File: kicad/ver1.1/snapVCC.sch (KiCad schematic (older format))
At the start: 16 parts, among them J1 Jumper Shunt, P1 CONN_01X03, P2 CONN_01X02, Q1 IRLML9301TRPbF, U1 TPS560200

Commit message: updated PCB
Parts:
- P1: footprint snapVCC_lib:3P-1.27 -> Connect:PINHEAD1-3
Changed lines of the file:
@@
 LIBS:contrib
 LIBS:valves
-LIBS:snapVCC
-LIBS:snapVCC-cache
+LIBS:bb
+LIBS:blinky-cache
 EELAYER 25 0
 EELAYER END
@@
 F 0 "P1" H 7000 4900 50  0000 C CNN
 F 1 "CONN_01X03" V 7100 4700 50  0001 C CNN
-F 2 "snapVCC_lib:3P-1.27" H 7000 4700 60  0001 C CNN
+F 2 "Connect:PINHEAD1-3" H 7000 4700 60  0001 C CNN
 F 3 "" H 7000 4700 60  0000 C CNN
 F 4 "1.27 mm pitch, male" H 7000 4700 60  0001 C CNN "Characteristics"

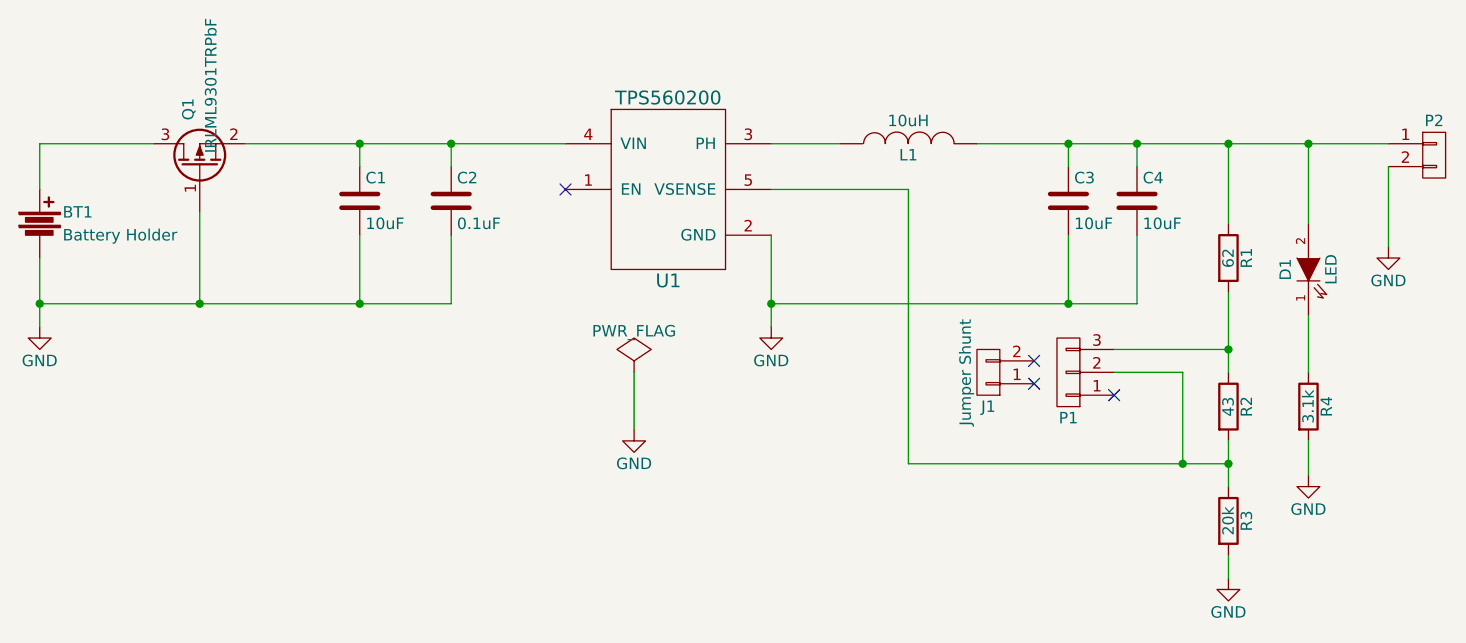
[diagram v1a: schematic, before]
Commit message: updated PCB
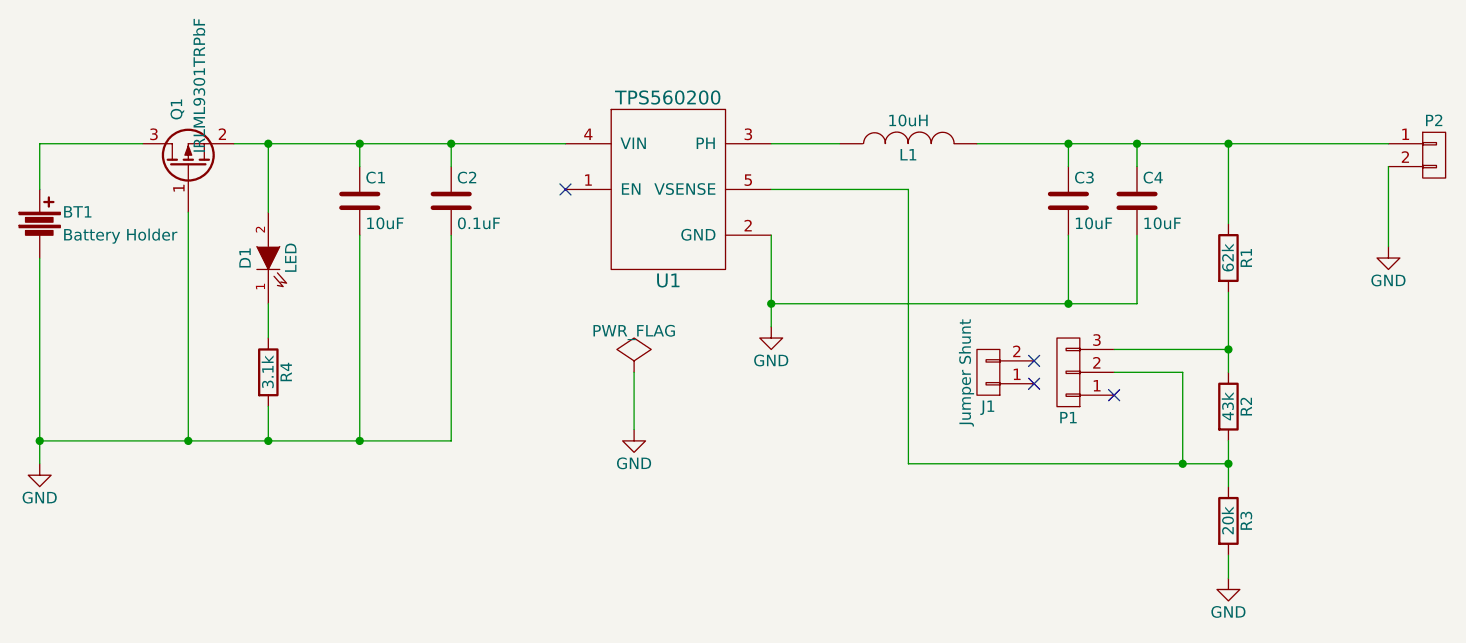
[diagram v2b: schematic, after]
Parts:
- R1: value 62 -> 62k
- R2: value 43 -> 43k
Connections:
- net at C1.1, C2.1, Q1.2 (S)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: now also D1.2 (A)
- net at C3.1, C4.1, L1.2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: no longer D1.2 (A)
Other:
- moved on the sheet: D1, Q1, R4
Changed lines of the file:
@@
 LIBS:contrib
 LIBS:valves
-LIBS:bb
-LIBS:blinky-cache
+LIBS:snapVCC
+LIBS:snapVCC-cache
 EELAYER 25 0
 EELAYER END
@@
 L Q_PMOS_GSD Q1
 U 1 1 56012F07
-P 3200 3800
-F 0 "Q1" H 3500 3850 50  0000 R CNN
-F 1 "IRLML9301TRPbF" H 3850 3750 50  0000 R CNN
-F 2 "snapVCC_lib:SOT23" H 3400 3900 29  0001 C CNN
-F 3 "" H 3200 3800 60  0000 C CNN
-F 4 "International Rectifier" H 3200 3800 60  0001 C CNN "MFN"
-F 5 "IRLML9301TRPbF" H 3200 3800 60  0001 C CNN "MFP"
-F 6 "Value" H 3200 3800 60  0001 C CNN "Link1"
-	1    3200 3800
+P 3150 3800
+F 0 "Q1" H 3450 3850 50  0000 R CNN
+F 1 "IRLML9301TRPbF" H 3800 3750 50  0000 R CNN
+F 2 "snapVCC_lib:SOT23" H 3350 3900 29  0001 C CNN
+F 3 "" H 3150 3800 60  0000 C CNN
+F 4 "International Rectifier" H 3150 3800 60  0001 C CNN "MFN"
+F 5 "IRLML9301TRPbF" H 3150 3800 60  0001 C CNN "MFP"
+F 6 "Value" H 3150 3800 60  0001 C CNN "Link1"
+	1    3150 3800
 	0    -1   -1   0
 $EndComp
@@
 P 7700 4200
 F 0 "R1" V 7780 4200 50  0000 C CNN
-F 1 "62" V 7700 4200 50  0000 C CNN
+F 1 "62k" V 7700 4200 50  0000 C CNN
 F 2 "snapVCC_lib:0603-RES" V 7630 4200 30  0001 C CNN
 F 3 "" H 7700 4200 30  0000 C CNN
@@
 P 7700 4850
 F 0 "R2" V 7780 4850 50  0000 C CNN
-F 1 "43" V 7700 4850 50  0000 C CNN
+F 1 "43k" V 7700 4850 50  0000 C CNN
 F 2 "snapVCC_lib:0603-RES" V 7630 4850 30  0001 C CNN
 F 3 "" H 7700 4850 30  0000 C CNN
@@
 L GND #PWR02
 U 1 1 56014277
-P 2500 4500
-F 0 "#PWR02" H 2500 4250 50  0001 C CNN
-F 1 "GND" H 2500 4350 50  0000 C CNN
-F 2 "" H 2500 4500 60  0000 C CNN
-F 3 "" H 2500 4500 60  0000 C CNN
-	1    2500 4500
+P 2500 5100
+F 0 "#PWR02" H 2500 4850 50  0001 C CNN
+F 1 "GND" H 2500 4950 50  0000 C CNN
+F 2 "" H 2500 5100 60  0000 C CNN
+F 3 "" H 2500 5100 60  0000 C CNN
+	1    2500 5100
 	1    0    0    -1
 $EndComp
@@
 $EndComp
 NoConn ~ 7200 4800
-Connection ~ 3200 4400
-Wire Wire Line
-	3200 4000 3200 4400
+Connection ~ 3150 5000
+Wire Wire Line
+	3150 4000 3150 5000
 Wire Wire Line
 	5100 4700 5100 4950
@@
 Wire Wire Line
 	5700 3700 6000 3700
-Connection ~ 3900 4400
-Wire Wire Line
-	4300 4400 4300 4100
-Connection ~ 2500 4400
-Wire Wire Line
-	3900 4400 3900 4100
-Wire Wire Line
-	2500 4400 4300 4400
+Connection ~ 3900 5000
+Wire Wire Line
+	4300 5000 4300 4100
+Connection ~ 2500 5000
+Wire Wire Line
+	3900 5000 3900 4100
+Wire Wire Line
+	2500 5000 4300 5000
 Connection ~ 4300 3700
 Wire Wire Line
@@
 	3900 3800 3900 3700
 Wire Wire Line
-	3400 3700 4800 3700
-Wire Wire Line
-	2500 3700 3000 3700
+	3350 3700 4800 3700
+Wire Wire Line
+	2500 3700 2950 3700
 Wire Wire Line
 	2500 3900 2500 3700
 Wire Wire Line
-	2500 4200 2500 4500
+	2500 4200 2500 5100
 Wire Wire Line
 	5700 4100 5700 4500
@@
 L R R4
 U 1 1 56016631
-P 8050 4850
-F 0 "R4" V 8130 4850 50  0000 C CNN
-F 1 "3.1k" V 8050 4850 50  0000 C CNN
-F 2 "Resistors_SMD:R_0402" V 7980 4850 30  0001 C CNN
-F 3 "" H 8050 4850 30  0000 C CNN
-F 4 "Resistor, Chip, 1/16W, 1%" H 8050 4850 60  0001 C CNN "Characteristics"
-F 5 "0402" H 8050 4850 60  0001 C CNN "Package ID"
-F 6 "Value" H 8050 4850 60  0001 C CNN "Link1"
-	1    8050 4850
+P 3500 4700
+F 0 "R4" V 3580 4700 50  0000 C CNN
+F 1 "3.1k" V 3500 4700 50  0000 C CNN
+F 2 "Resistors_SMD:R_0402" V 3430 4700 30  0001 C CNN
+F 3 "" H 3500 4700 30  0000 C CNN
+F 4 "Resistor, Chip, 1/16W, 1%" H 3500 4700 60  0001 C CNN "Characteristics"
+F 5 "0402" H 3500 4700 60  0001 C CNN "Package ID"
+F 6 "Value" H 3500 4700 60  0001 C CNN "Link1"
+	1    3500 4700
 	1    0    0    -1
 $EndComp
@@
 L LED D1
 U 1 1 56016668
-P 8050 4250
-F 0 "D1" H 8050 4350 50  0000 C CNN
-F 1 "LED" H 8050 4150 50  0000 C CNN
-F 2 "snapVCC_lib:LED-0603" H 8050 4250 60  0001 C CNN
-F 3 "" H 8050 4250 60  0000 C CNN
-F 4 "ROHM" H 8050 4250 60  0001 C CNN "MFN"
-F 5 "SML-P11MT" H 8050 4250 60  0001 C CNN "MFP"
-F 6 "Value" H 8050 4250 60  0001 C CNN "Link1"
-	1    8050 4250
+P 3500 4200
+F 0 "D1" H 3500 4300 50  0000 C CNN
+F 1 "LED" H 3500 4100 50  0000 C CNN
+F 2 "snapVCC_lib:LED-0603" H 3500 4200 60  0001 C CNN
+F 3 "" H 3500 4200 60  0000 C CNN
+F 4 "ROHM" H 3500 4200 60  0001 C CNN "MFN"
+F 5 "SML-P11MT" H 3500 4200 60  0001 C CNN "MFP"
+F 6 "Value" H 3500 4200 60  0001 C CNN "Link1"
+	1    3500 4200
 	0    -1   -1   0
 $EndComp
-Wire Wire Line
-	8050 3700 8050 4050
-Connection ~ 8050 3700
-Wire Wire Line
-	8050 4450 8050 4700
-$Comp
-L GND #PWR07
-U 1 1 56016795
-P 8050 5150
-F 0 "#PWR07" H 8050 4900 50  0001 C CNN
-F 1 "GND" H 8050 5000 50  0000 C CNN
-F 2 "" H 8050 5150 60  0000 C CNN
-F 3 "" H 8050 5150 60  0000 C CNN
-	1    8050 5150
-	1    0    0    -1
-$EndComp
-Wire Wire Line
-	8050 5000 8050 5150
 Connection ~ 5700 4400
 Connection ~ 7000 4400
@@
 NoConn ~ 6850 4650
 NoConn ~ 6850 4750
+Wire Wire Line
+	3500 4000 3500 3700
+Connection ~ 3500 3700
+Wire Wire Line
+	3500 4850 3500 5000
+Connection ~ 3500 5000
+Wire Wire Line
+	3500 4400 3500 4550
 $EndSCHEMATC
